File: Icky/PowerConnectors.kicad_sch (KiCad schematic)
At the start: 28 parts, among them J1 XT60PW-M, J11 XT30AW-M, J13 XT30AW-M, J14 XT30AW-M, J17 XT30UPB-F, J2 XT60PW-F, J3 XT30PW-F, J5 XT30PW-F, J6 XT30PW-F, J7 XT30UPB-F, J8 XT30UPB-F

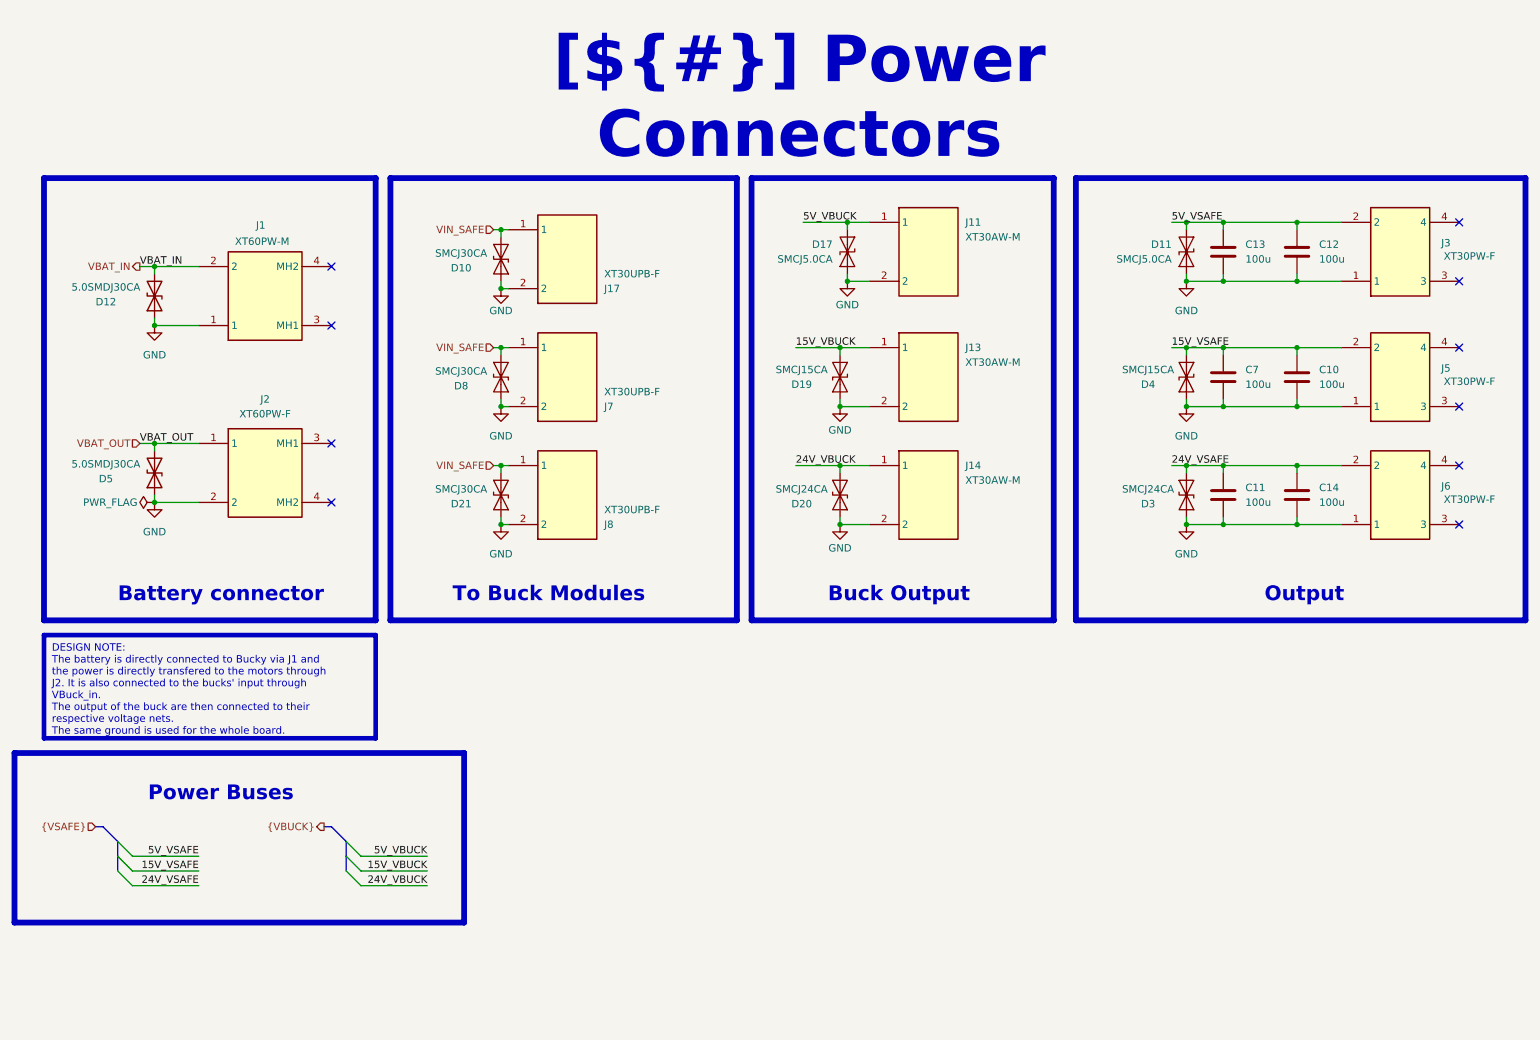
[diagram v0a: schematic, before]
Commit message: ERC passed v2
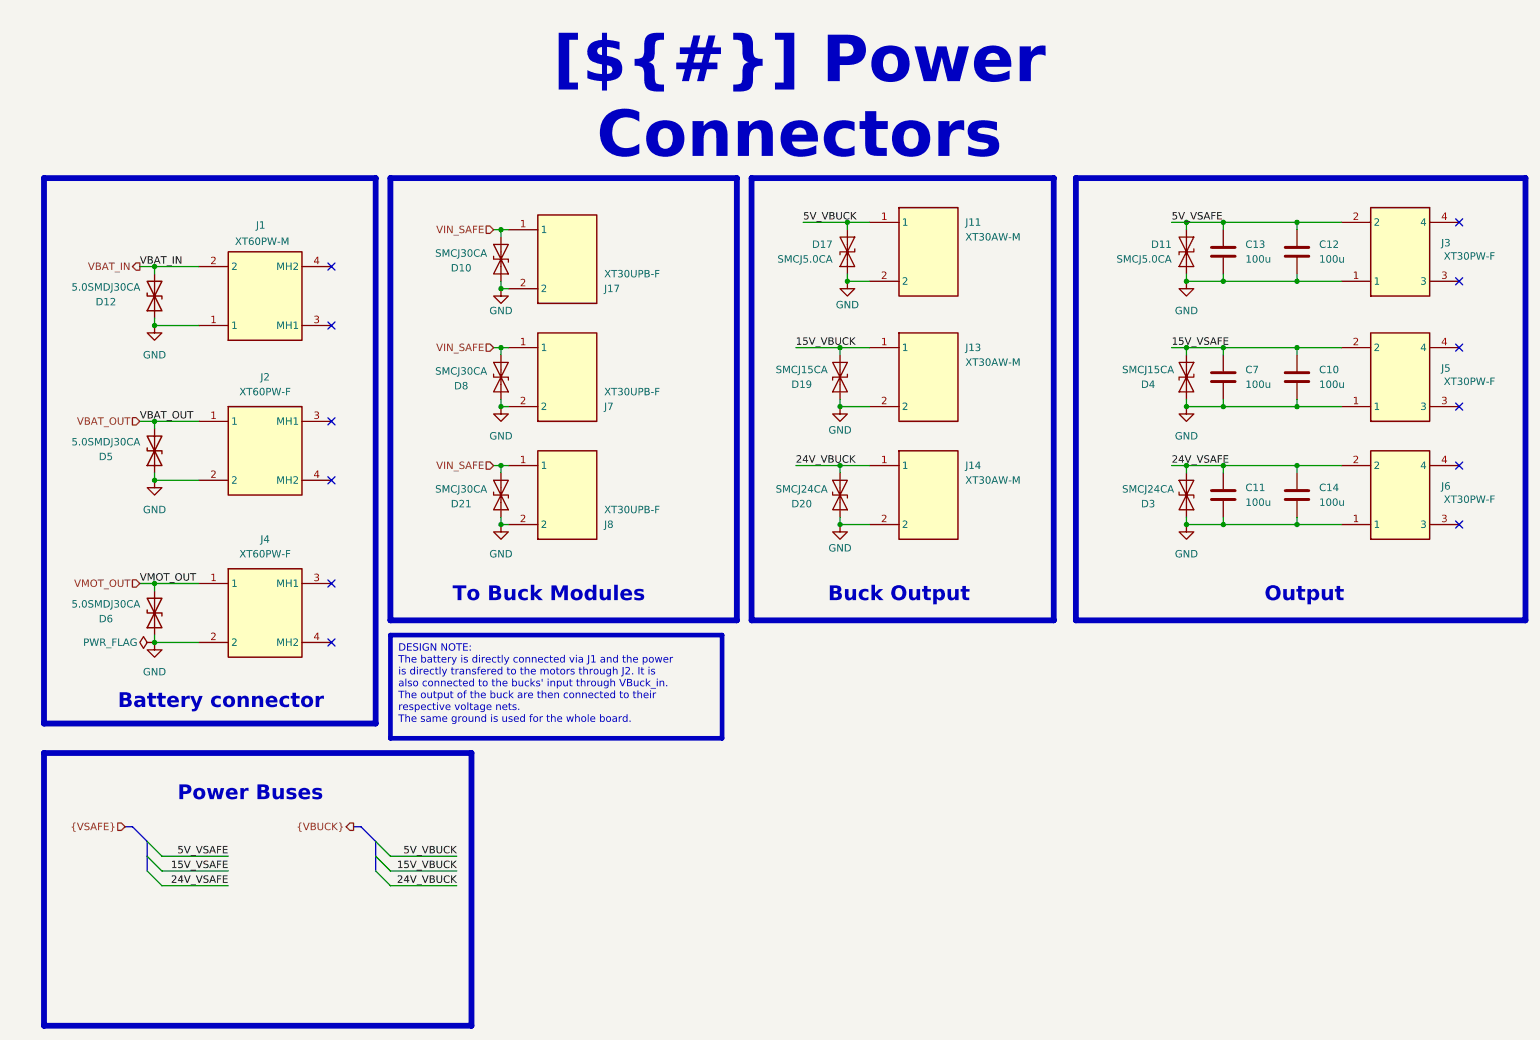
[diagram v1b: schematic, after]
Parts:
- added D6: 5.0SMDJ30CA, DIONM7959X262N, symbol Device:D_TVS
- added J4: XT60PW-F, XT60PWF, symbol SamacSys_Parts:XT60PW-F
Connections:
- net GND: now also D6.1 (A1), J4.2
- new net VMOT_OUT: D6.2 (A2), J4.1
- no-connect marks 10 -> 12
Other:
- moved on the sheet: D5, J2
